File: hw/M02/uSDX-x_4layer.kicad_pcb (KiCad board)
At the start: 4 copper layers, 100 x 89.8 mm, 89 parts, among them J1 DC Jack, J10 1602LCD, J11 PJ-324M, J12 PJ-324M, J13 PA MOSFETs, J2 FilterConn, J3 Antenna, J4 Etherkit si5351, J5 EK CLK0, J6 EK CLK1, J7 EK CLK2, J8 Adafruit si5351, J9 SSD1306 OLED and I2C out, Q1 S9013, Q2 S9013, Q3 S9012, Q4 2N7002, Q5 IRLML2060, SW1 SW_DPDT_x2, SW2 L, SW3 R, SW4 Rotary Encoder, U1 SN74CBT3253PWR, U2 NE5532DR

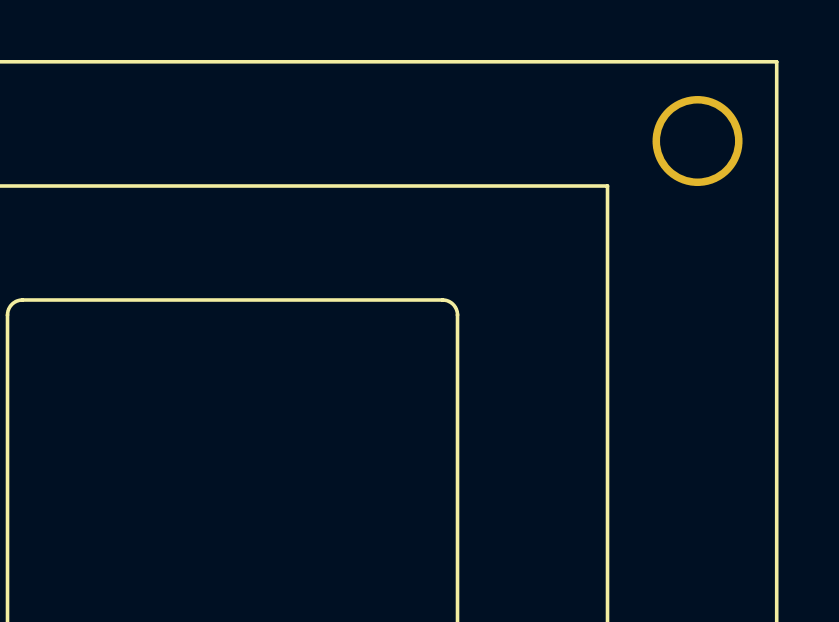
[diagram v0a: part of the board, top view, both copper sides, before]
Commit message: Early board development and CAT investigation
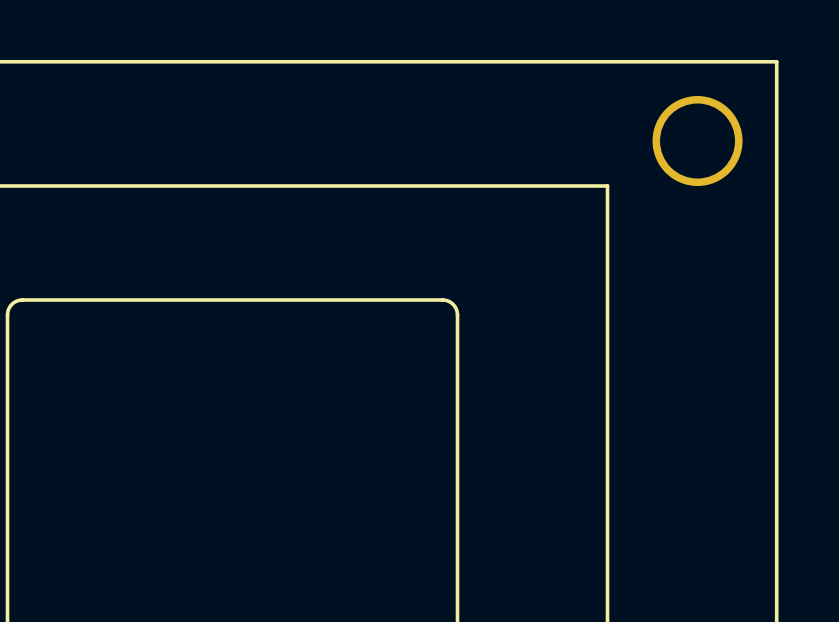
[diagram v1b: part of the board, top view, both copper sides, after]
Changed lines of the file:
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@@
     (fp_arc (start 63.7 8) (mid 64.053553 8.146447) (end 64.2 8.5)
       (stroke (width 0.12) (type solid)) (layer "F.SilkS"))
-    (fp_arc (start 64.20104 22.49932) (mid 64.054479 22.85315) (end 63.70066 22.9997)
+    (fp_arc (start 64.20104 22.49932) (mid 64.054473 22.853115) (end 63.70066 22.9997)
       (stroke (width 0.12) (type solid)) (layer "F.SilkS"))
     (fp_line (start -8.25 -2.75) (end -8.25 33.75)
@@
   (gr_line (start 189.35 53.4) (end 189.35 143.15)
     (stroke (width 0.05) (type solid)) (layer "Edge.Cuts"))
+  (dimension (type aligned) (layer "F.Cu")
+    (pts (xy 187.96 53.34) (xy 91.44 53.34))
+    (height 7.62)
+    (gr_text "96.5200 mm" (at 139.7 43.92) (layer "F.Cu")
+      (effects (font (size 1.5 1.5) (thickness 0.3)))
+    )
+    (format (prefix "") (suffix "") (units 3) (units_format 1) (precision 4))
+    (style (thickness 0.2) (arrow_length 1.27) (text_position_mode 0) (extension_height 0.58642) (extension_offset 0.5) keep_text_aligned)
+  )
+  (dimension (type aligned) (layer "F.Cu")
+    (pts (xy 91.44 53.34) (xy 91.44 142.24))
+    (height 10.159999)
+    (gr_text "88.9000 mm" (at 79.480001 97.79 90) (layer "F.Cu")
+      (effects (font (size 1.5 1.5) (thickness 0.3)))
+    )
+    (format (prefix "") (suffix "") (units 3) (units_format 1) (precision 4))
+    (style (thickness 0.2) (arrow_length 1.27) (text_position_mode 0) (extension_height 0.58642) (extension_offset 0.5) keep_text_aligned)
+  )
   (dimension (type aligned) (layer "Dwgs.User")
     (pts (xy 189.35 52.9) (xy 89.35 52.9))
